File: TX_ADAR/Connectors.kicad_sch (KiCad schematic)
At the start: 8 parts, among them J1 Conn_Coaxial, J11 RJ45_LED_Shielded, J12 RJ45_LED_Shielded, J13 Conn_Coaxial, J14 Conn_Coaxial, J15 FX8-120S-SV21, J16 RJ45_LED_Shielded, J2 Conn_Coaxial

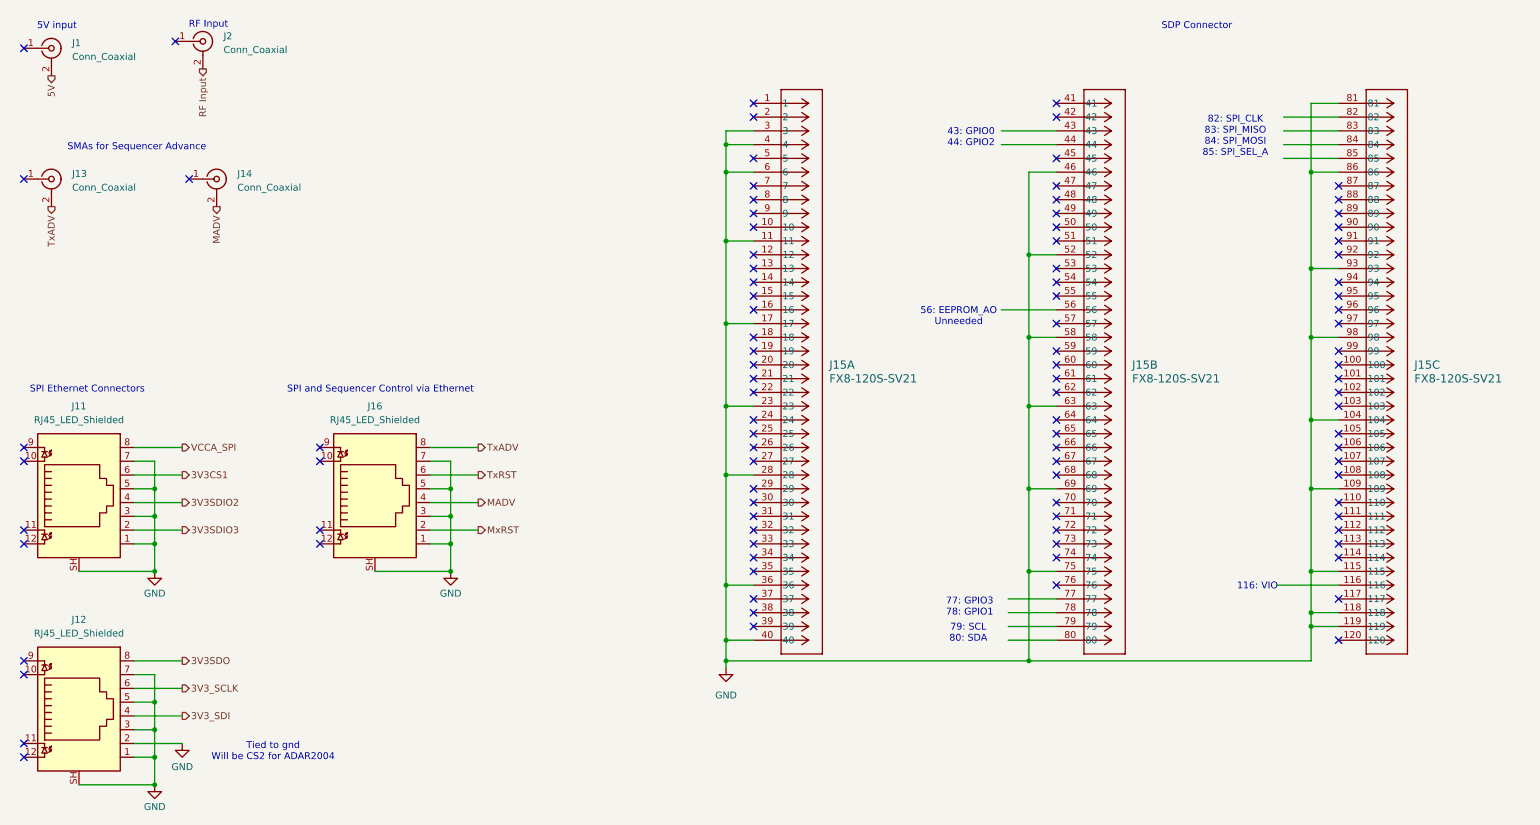
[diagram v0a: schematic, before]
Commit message: Moving things around
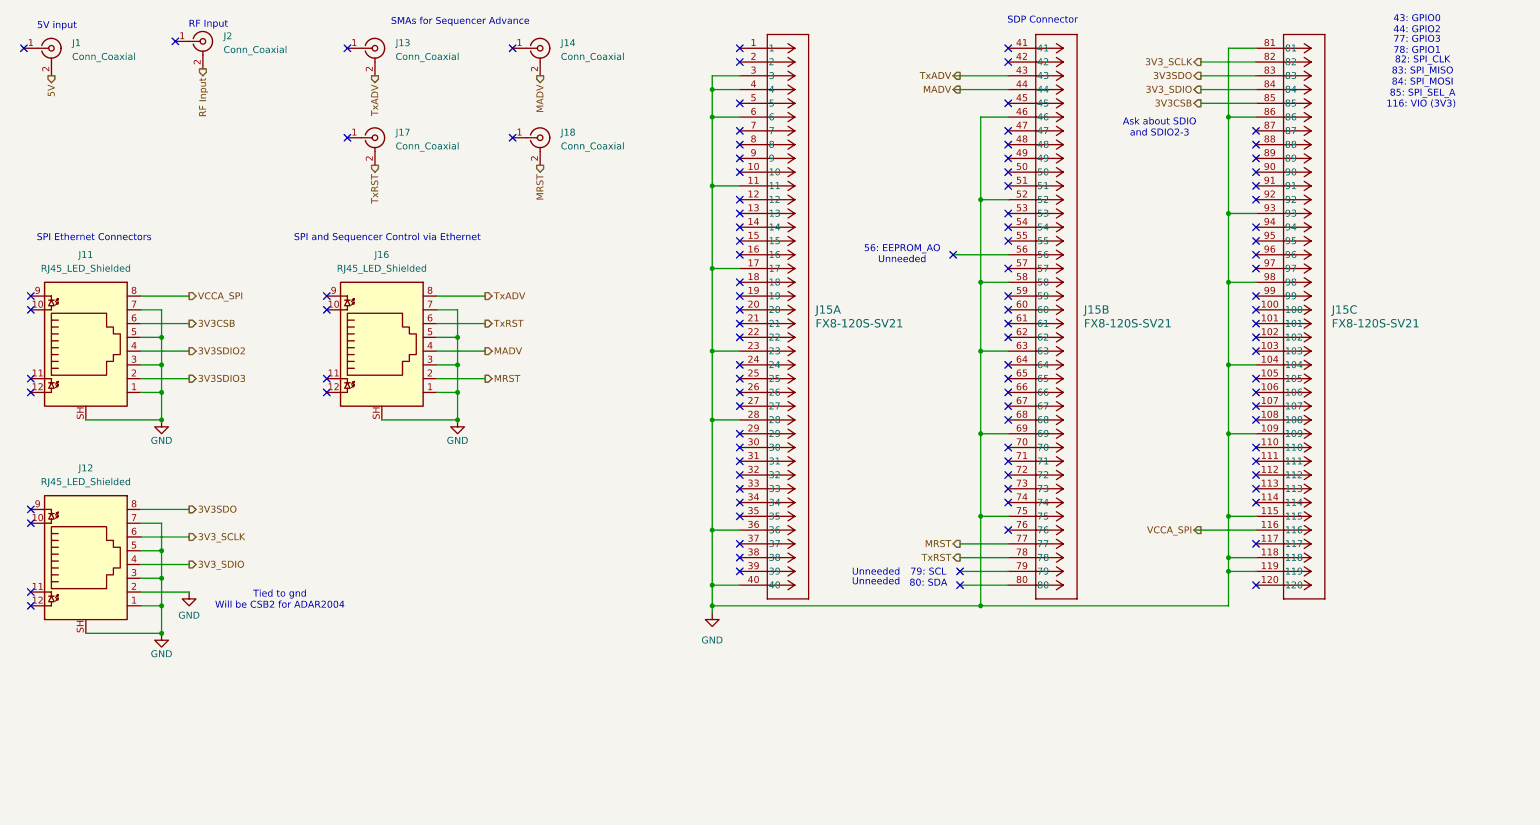
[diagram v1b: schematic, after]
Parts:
- added J17, J18: Conn_Coaxial, symbol Connector:Conn_Coaxial
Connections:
- net 3V3CS1 is gone; now on net 3V3CSB: J11.6
- net 3V3_SDI is gone; now on net 3V3_SDIO: J12.4
- net MxRST is gone; now on net MRST: J16.2
- net 3V3SDO: now also J15.83
- net 3V3_SCLK: now also J15.82
- net MADV: now also J15.44
- net TxADV: now also J15.43
- net TxRST: now also J15.78, J17.2 (Ext)
- net VCCA_SPI: now also J15.116
- net 3V3_SDIO: now reaches J15.84
- net 3V3CSB: now reaches J15.85
- net MRST: now reaches J15.77
- net MRST: now also J18.2 (Ext)
- no-connect marks 100 -> 105
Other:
- note added: "116: VIO (3V3)"
- note added: "Ask about SDIO and SDIO2-3"
- note added: "Tied to gnd Will be CSB2 for ADAR2004"
- note removed: "116: VIO"
- note removed: "Tied to gnd Will be CS2 for ADAR2004"
- moved on the sheet: J11, J12, J13, J14, J15A, J15B, J15C, J16
